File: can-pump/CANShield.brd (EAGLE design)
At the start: 130.8 x 85.1 mm, 110 parts, among them IC2 MC1525TT, IC3 QUAD_OPAMPD, J1 POWERPOLE_POWER25A_HORIZONTAL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, K1 G5LE, K2 G5LE, K3 G5LE, K4 G5LE, K5 G5LE, K6 G5LE, K7 G5LE, K8 G5LE, Q1 MOSFET-NCHANNELAO3404A, Q2 MOSFET-NCHANNELAO3404A, Q3 MOSFET-NCHANNELAO3404A, Q4 MOSFET-NCHANNELAO3404A, Q5 MOSFET-NCHANNELAO3404A, Q6 MOSFET-NCHANNELAO3404A, Q7 MOSFET-NCHANNELAO3404A, Q8 MOSFET-NCHANNELAO3404A, U5 MCP2551, X2 SMKDSP_1,5/2, X5 SMKDSP_1,5/2, X6 SMKDSP_1,5/2, X7 SMKDSP_1,5/2, X8 SMKDSP_1,5/2

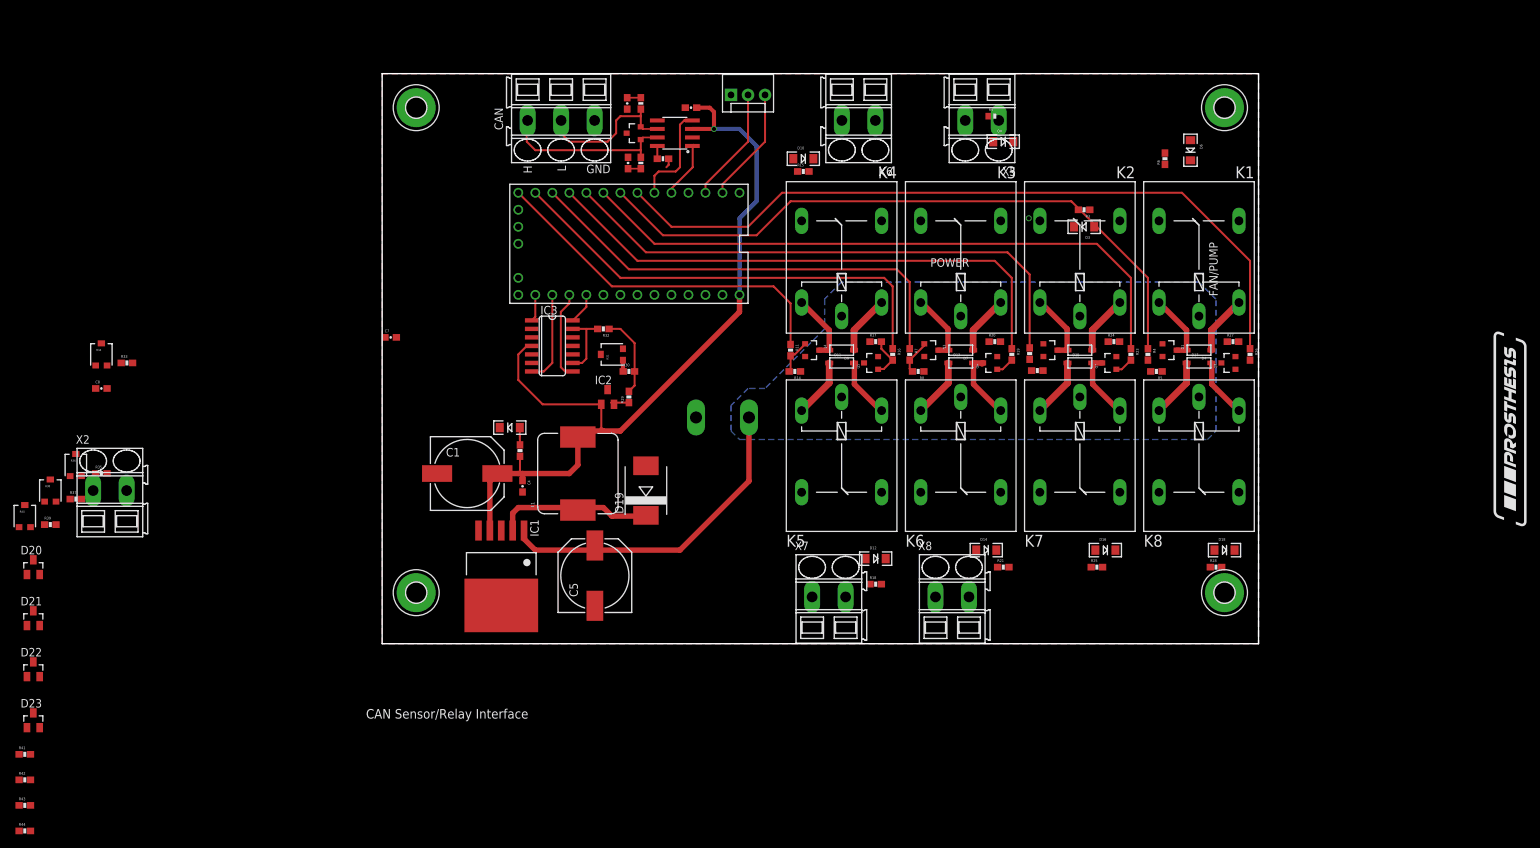
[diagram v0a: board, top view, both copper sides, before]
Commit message: Latest
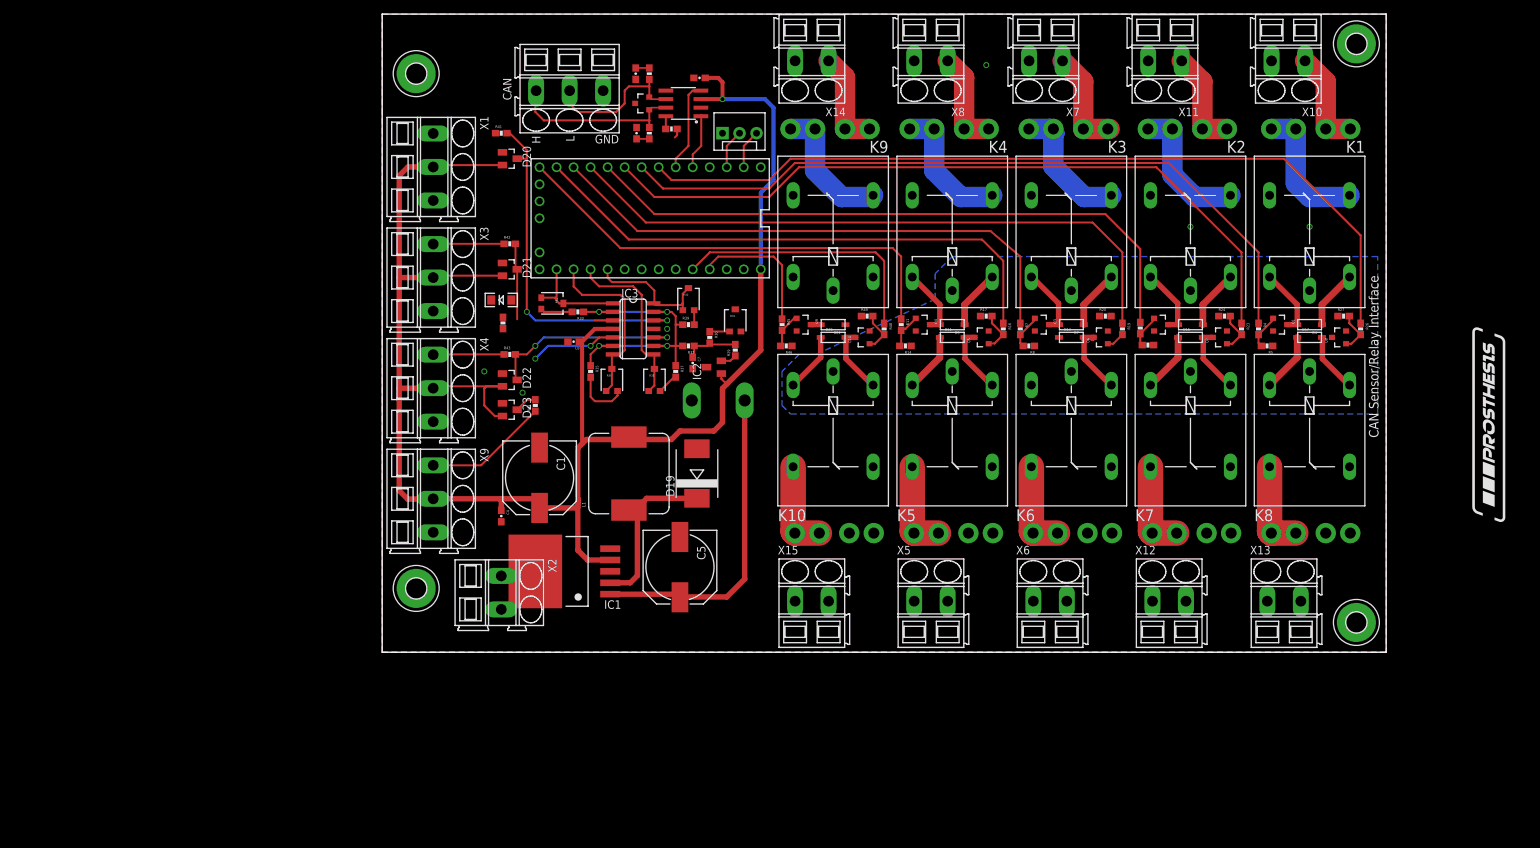
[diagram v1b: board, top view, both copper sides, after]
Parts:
- removed D10, D12, D14, D16, D18, D3, D6, D8: (no value), SparkFun-LED:LED-1206
- removed R15, R18, R21, R25, R28, R3, R6, R9: 1K, SparkFun-Passives:0603-RES
- added D24, D26: (no value), adafruit:SOD-123
- added K10, K9: G5LE, relay:G5LE
- added Q10, Q9: MOSFET-NCHANNELAO3404A, SparkFun-DiscreteSemi:SOT23-3
- added R45, R48: 100R, SparkFun-Passives:0603-RES
- added R46, R49: 10K, SparkFun-Passives:0603-RES
- added U$10, U$11, U$12, U$2, U$4, U$5, U$6, U$7, U$8, U$9: FUSE, grant:MINIFUSE
- added X1, X3, X4, X9: SMKDSP_1,5/3, con-phoenix-smkdsp:SMKDSP_1,5/3
- added X10, X11, X12, X13, X14, X15: SMKDSP_1,5/2, con-phoenix-smkdsp:SMKDSP_1,5/2
- moved R41 116.8 mm to (17.8, 73.7)
- moved R42 107.9 mm to (19.1, 57.1)
- moved R40 104.2 mm to (45.7, 48.9)
- moved R39 99.8 mm to (45.7, 45.1)
- moved R44 99.2 mm to (22.9, 33.0), turned to 90 degrees
- moved R43 98.8 mm to (19.1, 40.6)
- moved D20 93.7 mm to (19.1, 69.8), turned to 270 degrees
- moved R38 91.7 mm to (40.6, 36.8)
- moved R37 91.5 mm to (43.8, 38.1), turned to 270 degrees
- moved D21 88.1 mm to (19.1, 53.3), turned to 270 degrees
- moved X7 86.3 mm to (99.1, 84.5), turned to 180 degrees
- moved D23 84.9 mm to (19.1, 32.4), turned to 270 degrees
- moved D22 83.2 mm to (19.1, 36.8), turned to 270 degrees
- moved R36 81.0 mm to (34.3, 36.8)
- moved X8 80.1 mm to (81.9, 84.5), turned to 180 degrees
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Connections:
- removed net 5V: D20.2, D21.2, D22.2, D23.2
- removed net N$11: D6.A, R6.1
- removed net N$17: D8.A, R9.1
- removed net N$21: D10.A, R15.1
- removed net N$25: D12.A, R18.1
- removed net N$29: D14.A, R21.1
- removed net N$33: D16.A, R25.1
- removed net N$37: D18.A, R28.1
- removed net N$5: D3.A, R3.1
- new net N$15: K6.S, U$9.A1, U$9.A2
- new net N$20: R44.1, X9.1
- new net N$24: R42.1, X3.1
- new net N$28: R43.1, X4.1
- new net N$3: K3.S, U$7.A1, U$7.A2
- new net N$32: R41.1, X1.1
- new net N$4: K4.S, U$8.A1, U$8.A2
- new net N$41: K2.S, U$4.A1, U$4.A2
- new net N$45: K8.S, U$5.A1, U$5.A2
- new net N$50: K7.S, U$2.A1, U$2.A2
- new net N$53: K1.S, U$6.A1, U$6.A2
- new net N$55: D24.A, K9.2, Q9.3
- new net N$57: Q9.1, R45.2, R46.2
- new net N$59: D26.A, K10.2, Q10.3
- new net N$60: Q10.1, R48.2, R49.2
- new net N$62: K9.S, U$11.A1, U$11.A2
- new net N$63: K10.S, U$12.A1, U$12.A2
- new net N$65: U$5.B1, U$5.B2, X13.1
- new net N$66: U$4.B1, U$4.B2, X11.1
- new net N$67: U$6.B1, U$6.B2, X10.1
- new net N$68: U$9.B1, U$9.B2, X6.1
- new net N$69: K5.S, U$10.A1, U$10.A2
- new net N$70: U$7.B1, U$7.B2, X7.1
- new net N$71: U$10.B1, U$10.B2, X5.1
- new net N$72: U$12.B1, U$12.B2, X15.1
- new net N$73: U$11.B1, U$11.B2, X14.1
- new net N$8: U$8.B1, U$8.B2, X8.1
- new net RELAY10: R48.1, U$1.22/A8
- new net RELAY9: R45.1, U$1.23/A9
- net +5V: now also D20.2, D21.2, D22.2, D23.2, X1.2, X3.2, X4.2, X9.2
- net GND: now also Q10.2, Q9.2, R46.1, R49.1, X1.3, X10.2, X11.2, X12.2, X13.2, X14.2, X15.2, X3.3, X4.3, X5.2, X6.2, X7.2, X8.2, X9.3
- net N$12: no longer D8.C
- net N$18: no longer D10.C
- net N$2: no longer D3.C
- net N$22: no longer D12.C
- net N$26: no longer D14.C
- net N$30: no longer D16.C
- net N$34: no longer D18.C
- net N$48: now also IC3.12; no longer IC3.3
- net N$51: now also IC3.3; no longer IC3.12
- net N$6: no longer D6.C
- net N$64: now also U$2.B1, U$2.B2, X12.1; no longer D13.C, K6.1
- net VCC: now also D13.C, D24.C, D26.C, K10.1, K10.P, K6.1, K9.1, K9.P; no longer R15.2, R18.2, R21.2, R25.2, R28.2, R3.2, R6.2, R9.2
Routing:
- net +5V: track 129.4 -> 268.6 mm
- net N$48: track 0.00 -> 53.1 mm, vias 0 -> 2
- net RELAY10: track 0.00 -> 39.5 mm
- net REF: track 10.4 -> 46.5 mm, vias 0 -> 4
- net N$56: track 0.00 -> 29.6 mm, vias 0 -> 2
- net N$47: track 0.00 -> 24.2 mm, vias 0 -> 2
- net N$53: track 0.00 -> 21.0 mm
- net RELAY9: track 0.00 -> 20.9 mm
- net N$41: track 0.00 -> 20.6 mm
- net N$3: track 0.00 -> 20.5 mm
- net N$4: track 0.00 -> 20.3 mm
- net N$62: track 0.00 -> 20.3 mm
- net N$20: track 0.00 -> 18.6 mm
- net RELAY1: track 94.6 -> 111.6 mm
- net N$70: track 0.00 -> 15.4 mm
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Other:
- board size 130.8 x 85.1 mm -> 149.9 x 95.2 mm
- board text removed: "FAN/PUMP"
- board text removed: "POWER"
